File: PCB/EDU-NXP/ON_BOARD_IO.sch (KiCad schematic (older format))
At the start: 64 parts, among them Q1 2N7000, Q10 2N7000, Q11 2N7000, Q12 2N7000, Q2 2N7000, Q3 2N7000, Q4 2N7000, Q5 2N7000, Q6 2N7000, Q7 2N7000, Q8 2N7000, Q9 2N7000, SW2 SW_PUSH, SW3 SW_PUSH, SW4 SW_PUSH, SW5 SW_PUSH

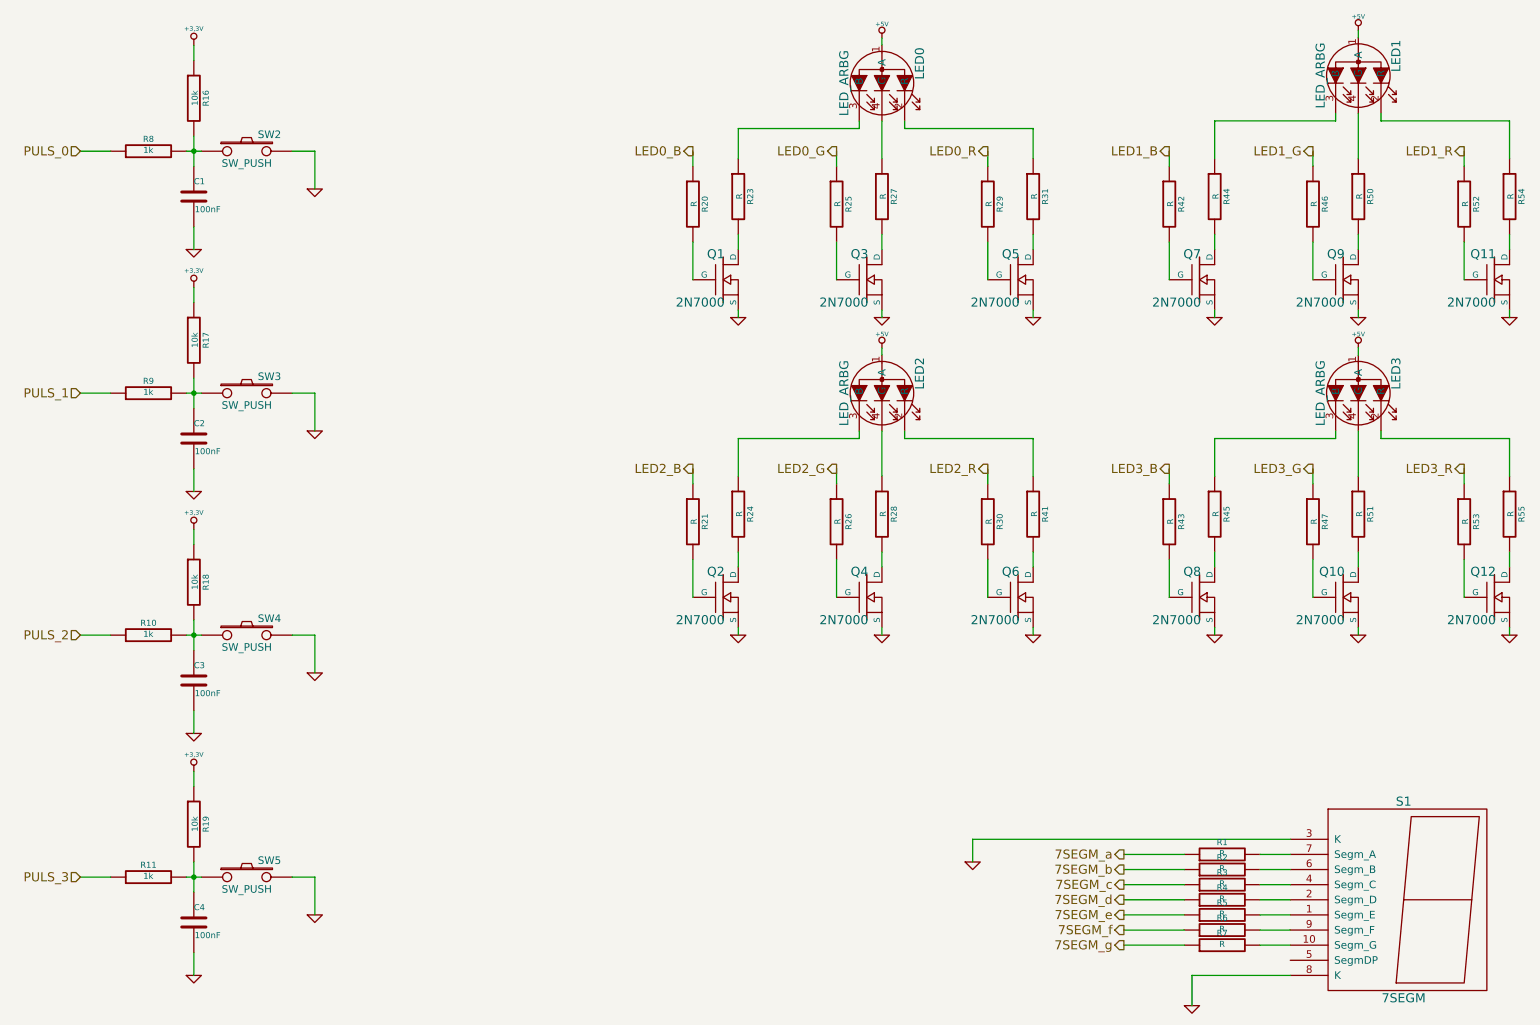
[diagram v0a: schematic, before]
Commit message: Primera versión
Primera versión de la EDU - CIAA
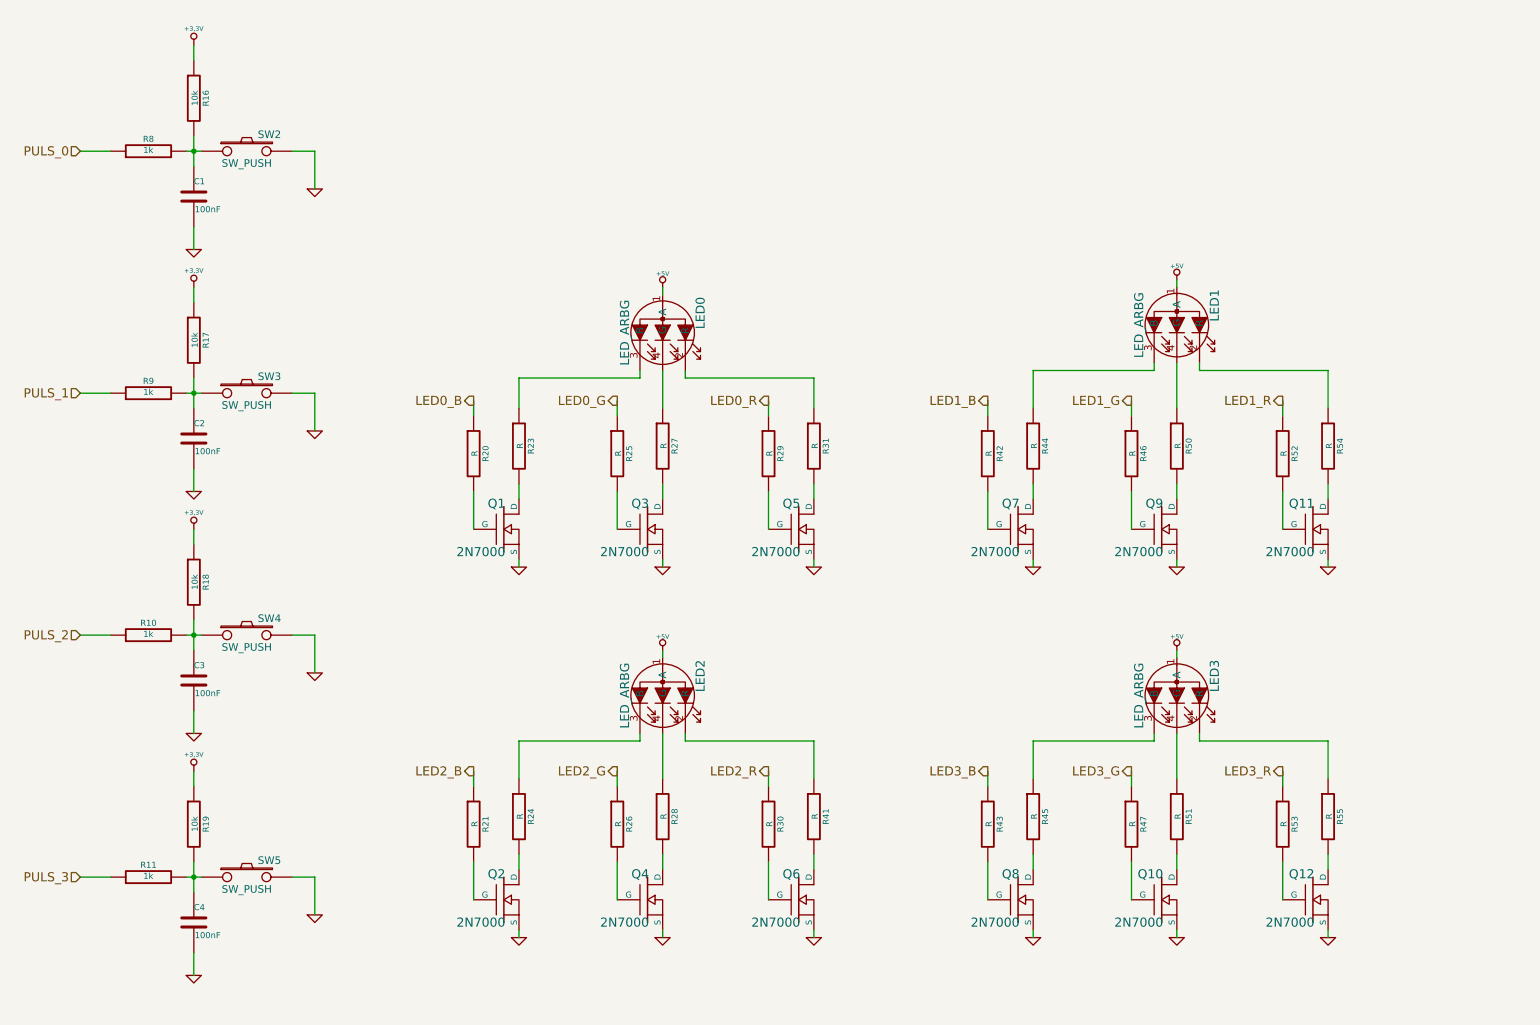
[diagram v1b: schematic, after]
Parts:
- removed R1, R2, R3, R4, R5, R6, R7: R, ~, symbol R
- removed S1: 7SEGM, ~, symbol 7SEGM
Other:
- moved on the sheet: LED0, LED1, LED2, LED3, Q1, Q10, Q11, Q12, Q2, Q3, Q4, Q5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
